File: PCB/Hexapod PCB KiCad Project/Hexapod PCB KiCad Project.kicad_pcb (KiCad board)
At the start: 2 copper layers, 96.5 x 96.5 mm, 34 parts, among them J1 Conn_01x03, J10 Conn_01x03, J11 Conn_01x03, J12 Conn_01x03, J13 Conn_01x03, J14 Conn_01x03, J15 Conn_01x03, J16 Conn_01x03, J17 Conn_01x03, J18 Conn_01x03, J19 Conn_01x03, J2 Battery, J20 Conn_01x03, J3 Conn_01x03, J4 Conn_01x03, J5 Switch, J6 Conn_01x03, J7 Conn_01x03, J8 Conn_01x03, J9 Conn_01x03, U1 DEV-16771, U2 Voltage Regulator, U3 NRF24L01_Breakout, U4 Gyro

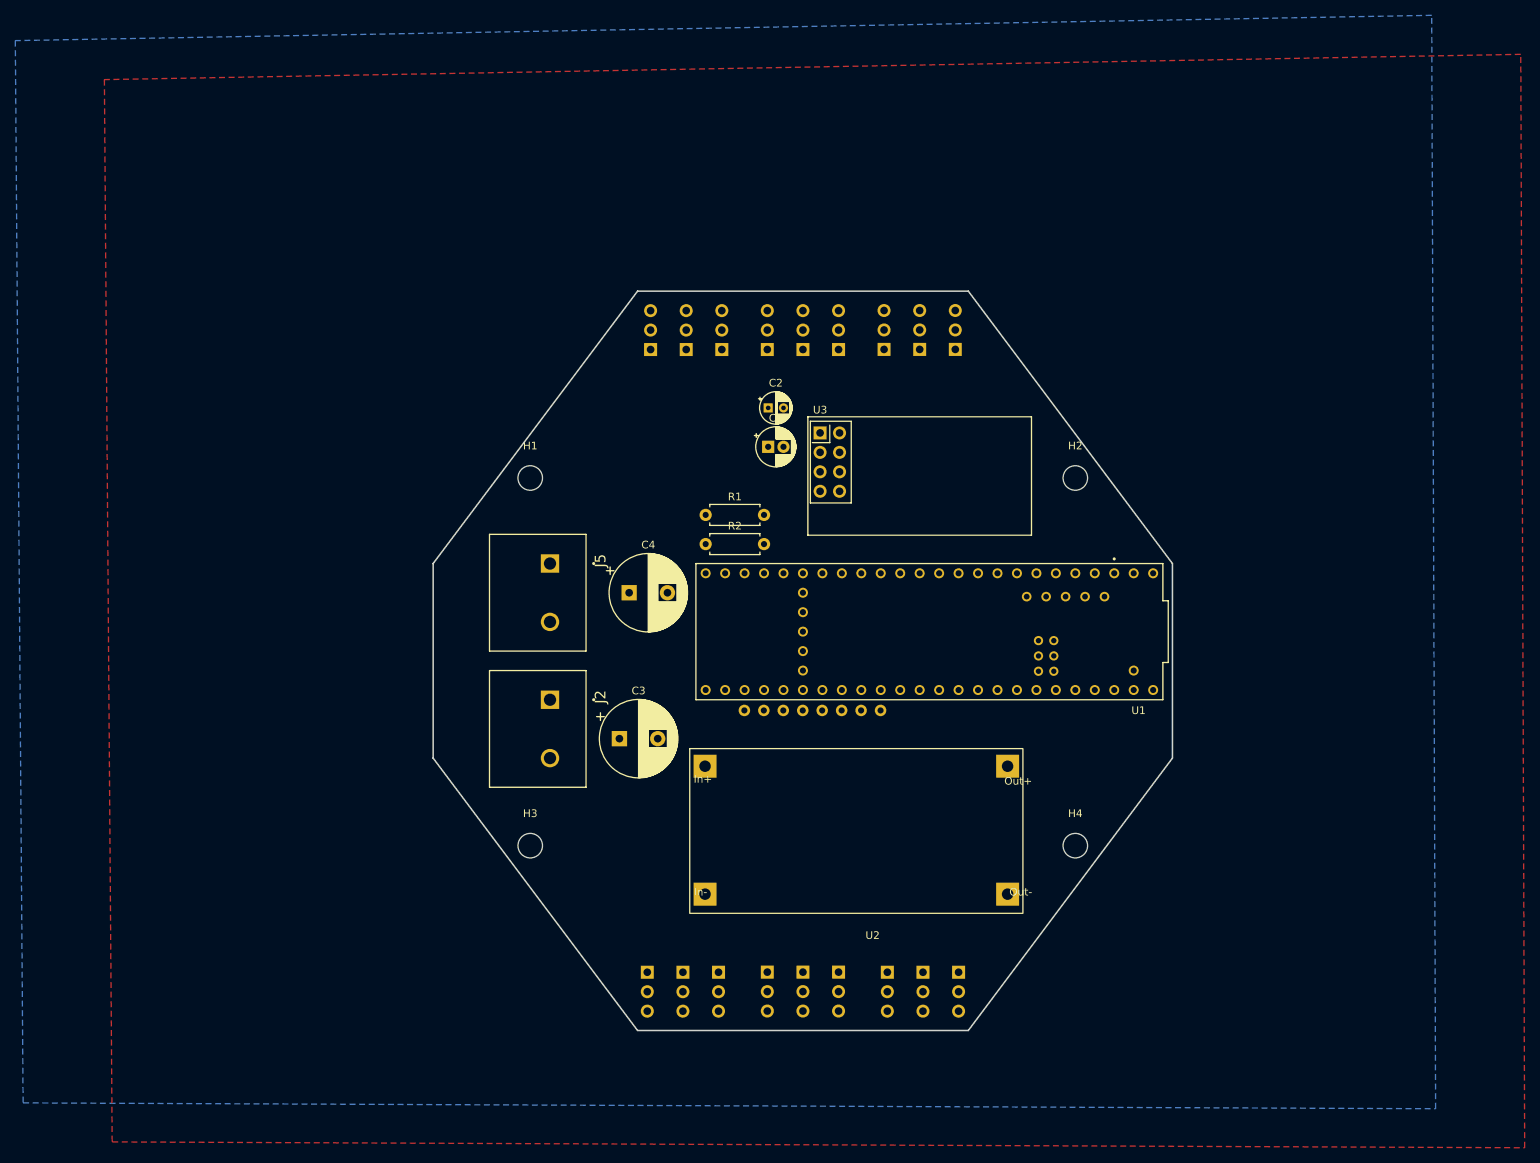
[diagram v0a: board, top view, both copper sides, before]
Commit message: traces
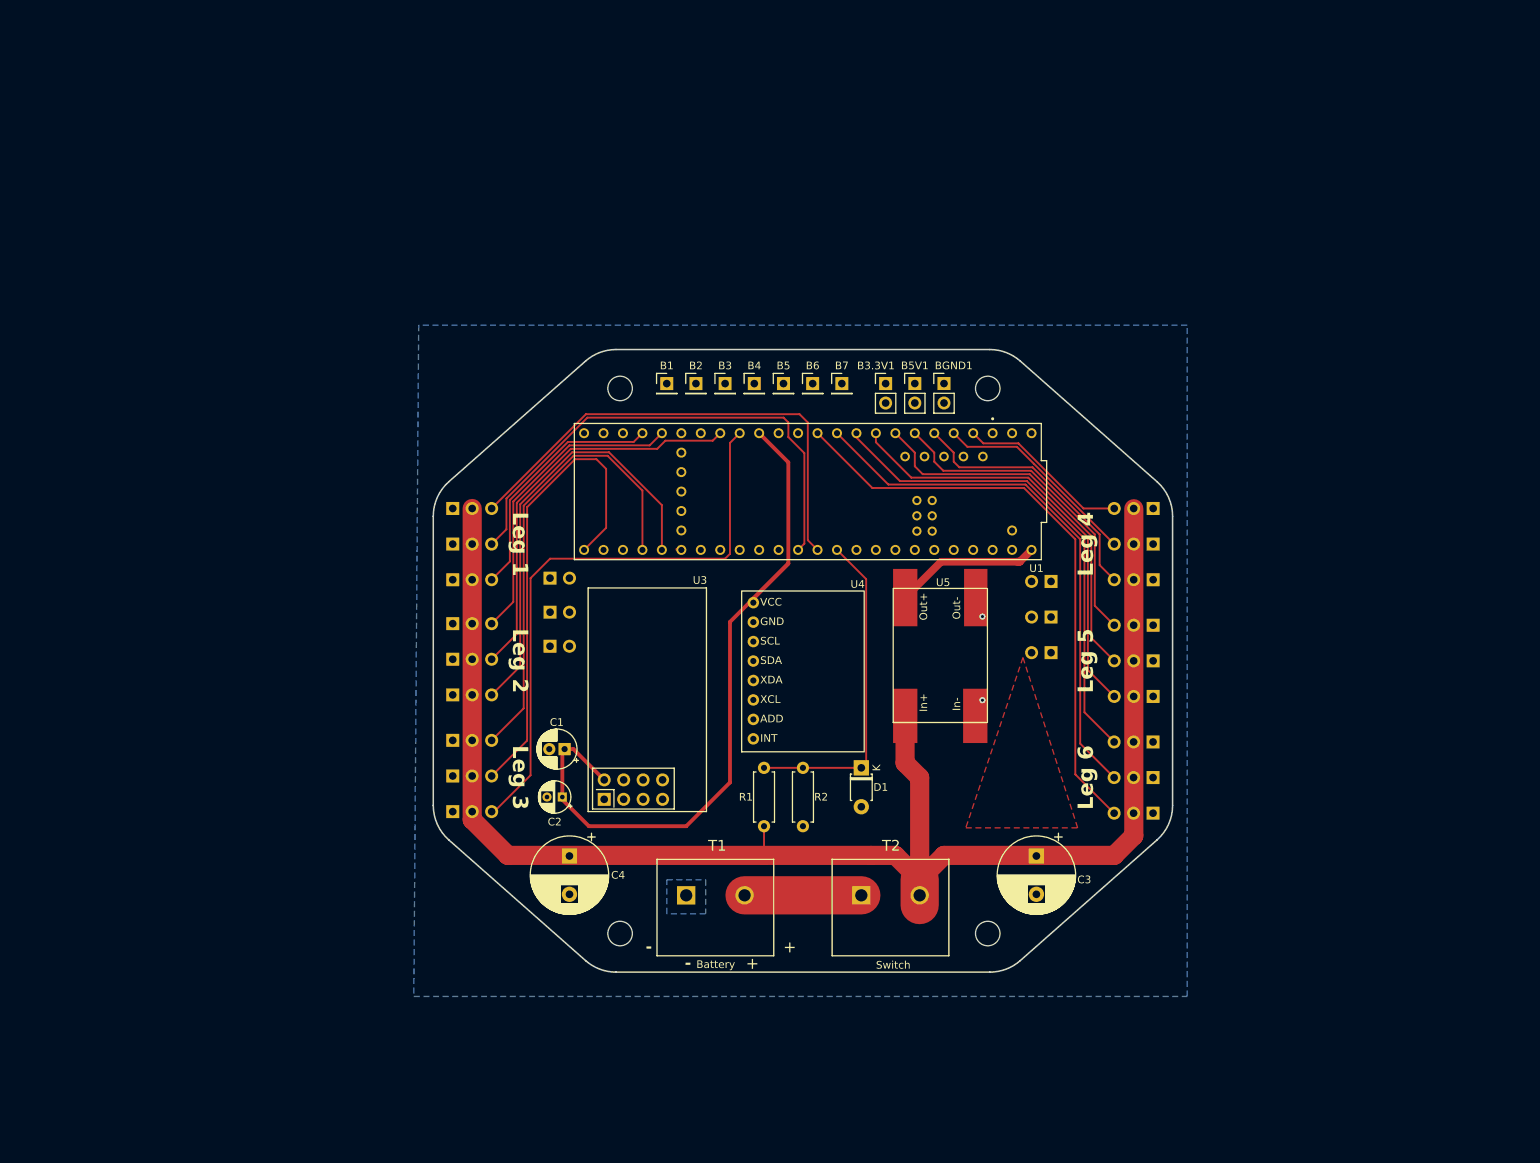
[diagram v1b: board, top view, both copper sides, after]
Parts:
- removed U2: Voltage Regulator, Voltage Regulator LM2596:Voltage Regulator LM2596
- added B1: Conn_01x01, Connector_PinHeader_2.54mm:PinHeader_1x01_P2.54mm_Vertical, F.Cu at (125.7, 65.4)
- added B2: Conn_01x01, Connector_PinHeader_2.54mm:PinHeader_1x01_P2.54mm_Vertical, F.Cu at (129.5, 65.4)
- added B3: Conn_01x01, Connector_PinHeader_2.54mm:PinHeader_1x01_P2.54mm_Vertical, F.Cu at (133.3, 65.4)
- added B3.3V1: Conn_01x02, Connector_PinHeader_2.54mm:PinHeader_1x02_P2.54mm_Vertical, F.Cu at (154.3, 65.4)
- added B4: Conn_01x01, Connector_PinHeader_2.54mm:PinHeader_1x01_P2.54mm_Vertical, F.Cu at (137.2, 65.4)
- added B5: Conn_01x01, Connector_PinHeader_2.54mm:PinHeader_1x01_P2.54mm_Vertical, F.Cu at (141.0, 65.4)
- added B5V1: Conn_01x02, Connector_PinHeader_2.54mm:PinHeader_1x02_P2.54mm_Vertical, F.Cu at (158.1, 65.4)
- added B6: Conn_01x01, Connector_PinHeader_2.54mm:PinHeader_1x01_P2.54mm_Vertical, F.Cu at (144.8, 65.4)
- added B7: Conn_01x01, Connector_PinHeader_2.54mm:PinHeader_1x01_P2.54mm_Vertical, F.Cu at (148.6, 65.4)
- added BGND1: Conn_01x02, Connector_PinHeader_2.54mm:PinHeader_1x02_P2.54mm_Vertical, F.Cu at (161.9, 65.4)
- added D1: D_Zener, Diode_THT:D_T-1_P5.08mm_Horizontal, F.Cu at (151.1, 115.6)
- added FS1: Foot Switch 1, Connector_PinHeader_2.54mm:PinHeader_1x02_P2.54mm_Vertical, B.Cu at (110.5, 90.8)
- added FS2: Foot Switch 2, Connector_PinHeader_2.54mm:PinHeader_1x02_P2.54mm_Vertical, B.Cu at (110.5, 95.2)
- added FS3: Foot Switch 3, Connector_PinHeader_2.54mm:PinHeader_1x02_P2.54mm_Vertical, B.Cu at (110.5, 99.7)
- added FS4: Foot Switch 4, Connector_PinHeader_2.54mm:PinHeader_1x02_P2.54mm_Vertical, B.Cu at (175.9, 91.2)
- added FS5: Foot Switch 5, Connector_PinHeader_2.54mm:PinHeader_1x02_P2.54mm_Vertical, B.Cu at (175.9, 95.9)
- added FS6: Foot Switch 6, Connector_PinHeader_2.54mm:PinHeader_1x02_P2.54mm_Vertical, B.Cu at (175.9, 100.5)
- added G***: LOGO, LOGO, F.Cu at (172.4, 113.9)
- added U5: Buck Converter 5V MP1584EN, Buck Converter 5V MP1584EN:Buck Converter 5V MP1584EN, F.Cu at (169.6, 100.9)
- R1: value 10k -> R1
- R2: value 22k -> R2
- U4: value Gyro -> Gyro MPU6050; moved to F.Cu
- moved Tib4 89.6 mm to (189.2, 81.7), turned to 90 degrees
- moved Fem4 83.0 mm to (189.2, 86.4), turned to 90 degrees
- moved Cox4 76.5 mm to (189.2, 91.0), turned to 90 degrees
- moved Tib1 72.2 mm to (97.8, 91.0), turned to -90 degrees
- moved Tib3 69.8 mm to (97.8, 121.3), turned to -90 degrees
- moved Tib5 67.7 mm to (189.2, 97.0), turned to 90 degrees
- moved Tib2 67.6 mm to (97.8, 106.0), turned to -90 degrees
- moved Fem1 66.0 mm to (97.8, 86.4), turned to -90 degrees
- moved Fem3 63.5 mm to (97.8, 116.6), turned to -90 degrees
- moved Fem5 61.2 mm to (189.2, 101.6), turned to 90 degrees
- moved Fem2 61.0 mm to (97.8, 101.4), turned to -90 degrees
- moved H3 60.8 mm to (167.6, 137.2), turned to 90 degrees
- moved H4 60.8 mm to (167.6, 66.0), turned to 90 degrees
- moved H1 60.6 mm to (119.6, 137.2), turned to 90 degrees
- moved H2 60.6 mm to (119.6, 66.0), turned to 90 degrees
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- renumbered J18 to Cox1, J15 to Cox2, J12 to Cox3, J9 to Cox4, J6 to Cox5, J1 to Cox6, J19 to Fem1, J16 to Fem2, J13 to Fem3, J10 to Fem4, J7 to Fem5, J3 to Fem6, J2 to T1, J5 to T2, J20 to Tib1, J17 to Tib2, J14 to Tib3, J11 to Tib4, J8 to Tib5, J4 to Tib6
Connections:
- U1 pad 10: Leg1 Tibia -> Leg1 Coxa
- U1 pad 17: unconnected-(U1-A3-Pad17) -> B6
- U1 pad 2: Leg3 Coxa -> Leg3 Tibia
- U1 pad 20: unconnected-(U1-A6-Pad20) -> B7
- U1 pad 21: unconnected-(U1-A7-Pad21) -> FS6
- U1 pad 22: unconnected-(U1-A8-Pad22) -> FS5
- U1 pad 23: unconnected-(U1-A9-Pad23) -> FS4
- U1 pad 25: Leg4 Femur -> Leg5 Femur
- U1 pad 28: Leg4 Coxa -> Leg5 Coxa
- U1 pad 29: Leg5 Tibia -> Leg6 Tibia
- U1 pad 30: unconnected-(U1-CRX3-Pad30) -> B2
- U1 pad 31: unconnected-(U1-CTX3-Pad31) -> B1
- U1 pad 33: Leg5 Femur -> Leg4 Femur
- U1 pad 34: unconnected-(U1-RX8-Pad34) -> FS1
- U1 pad 35: unconnected-(U1-TX8-Pad35) -> FS2
- U1 pad 36: Leg5 Coxa -> Leg4 Coxa
- U1 pad 37: Leg6 Tibia -> Leg5 Tibia
- U1 pad 38: unconnected-(U1-A14-Pad38) -> FS3
- U1 pad 39: unconnected-(U1-A15-Pad39) -> B3
- U1 pad 4: Leg3 Tibia -> Leg3 Coxa
- U1 pad 40: unconnected-(U1-A16-Pad40) -> B4
- U1 pad 41: unconnected-(U1-A17-Pad41) -> B5
- U1 pad 5: Leg2 Coxa -> Leg2 Tibia
- U1 pad 7: Leg2 Tibia -> Leg2 Coxa
- U1 pad 8: Leg1 Coxa -> Leg1 Tibia
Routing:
- net +BATT: track 0.00 -> 386.3 mm
- net +3.3V: track 0.00 -> 128.2 mm
- net Leg1 Coxa: track 0.00 -> 77.2 mm
- net Leg4 Tibia: track 0.00 -> 76.4 mm
- net Leg1 Femur: track 0.00 -> 70.4 mm
- net Leg6 Femur: track 0.00 -> 66.0 mm
- net Leg6 Coxa: track 0.00 -> 64.0 mm
- net Leg1 Tibia: track 0.00 -> 63.9 mm
- net Leg4 Femur: track 0.00 -> 62.2 mm
- net Leg4 Coxa: track 0.00 -> 60.2 mm
- net MOSI: track 0.00 -> 57.6 mm
- net Teensy VIN: track 0.00 -> 57.3 mm
- net Leg5 Tibia: track 0.00 -> 56.4 mm
- net Leg2 Coxa: track 0.00 -> 56.2 mm
- net MISO: track 0.00 -> 54.5 mm
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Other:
- board size 96.5 x 96.5 mm -> 96.5 x 81.3 mm
- copper layers 2 -> 4
- board text added: "+"
- board text added: "-"
- board text added: "Aecert Robotics"
- board text added: "Aecert's"
- board text added: "Battery"
- board text added: "Designed By:"
- board text added: "Hexapod"
- board text added: "Leg 1"
- board text added: "Leg 2"
- board text added: "Leg 3"
- board text added: "Leg 4"
- board text added: "Leg 5"
- board text added: "Leg 6"
- board text added: "Manufactured By:"
- board text added: "PCBWay"
- board text added: "Switch"
- board text added: "aecertrobotics.com"
- board text added: "pcbway.com"
